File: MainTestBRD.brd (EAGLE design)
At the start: 100 x 62.2 mm, 24 parts, among them J1 COMPUTER-PERIPHERAL-POWERVERT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, U1 ATMEGA128-SMD

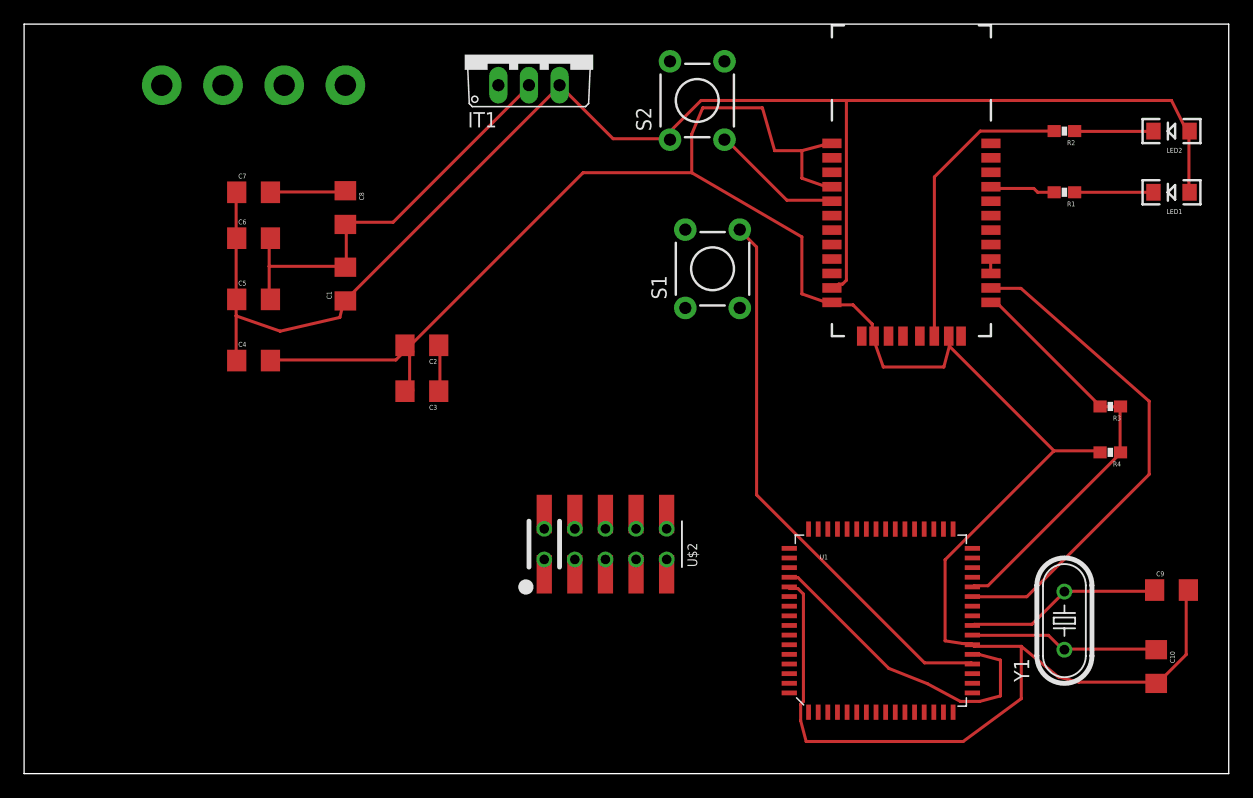
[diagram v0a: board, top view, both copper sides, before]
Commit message: other pinouts
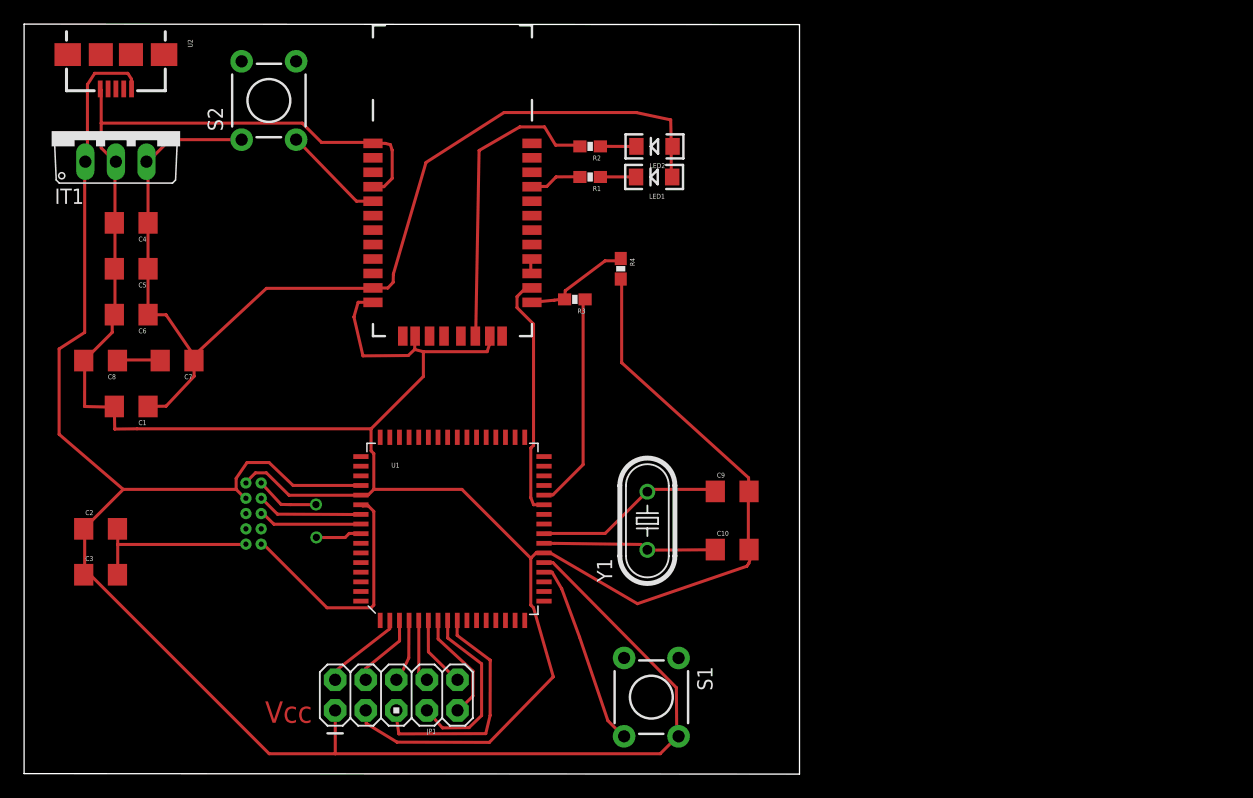
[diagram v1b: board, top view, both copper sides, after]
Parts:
- removed J1: COMPUTER-PERIPHERAL-POWERVERTICAL, SparkFun-Connectors:COMPUTER-PERIPHERAL-POWER
- removed U$2: JTAGICE3-CONNECTOR100MIL-SMD, con-jtagice3:JTAGICE3-100MIL-SMD
- added JP1: M05X2PTH, SparkFun-Connectors:AVR_ICSP
- added U$3: JTAGICE3-CONNECTOR50MIL-THT, con-jtagice3:JTAGICE3-50MIL
- added U2: (no value), SparkFun-Connectors:USB-AB-MICRO-SMD
- moved R3 45.3 mm to (45.7, 57.1)
- moved R4 43.4 mm to (49.5, 59.7), turned to 270 degrees
- moved LED1 43.0 mm to (52.3, 67.3)
- moved LED2 42.9 mm to (52.3, 69.8)
- moved R1 39.4 mm to (47.0, 67.3)
- moved R2 39.4 mm to (47.0, 69.8)
- moved U$1 38.1 mm to (35.6, 63.5)
- moved C9 37.4 mm to (58.8, 41.2)
- moved C10 36.5 mm to (58.8, 36.4), turned to 0 degrees
- moved U1 36.4 mm to (35.6, 38.1)
- moved S1 35.9 mm to (52.1, 24.1), turned to 270 degrees
- moved Y1 35.6 mm to (51.7, 38.8)
- moved S2 35.6 mm to (20.3, 73.7)
- moved IT1 34.9 mm to (7.62, 71.1)
- moved C2 30.7 mm to (6.35, 38.1), turned to 0 degrees
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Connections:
- new net N$10: JP1.10, U1.6
- new net N$11: JP1.8, U1.5
- new net N$12: JP1.6, U1.4
- new net N$13: JP1.4, U1.3
- new net N$14: JP1.2, U1.2
- new net N$15: JP1.9, U1.7
- new net N$16: JP1.7, U1.8
- new net N$17: JP1.5, U1.9
- new net N$3: R3.1, U1.28
- net BT_RX: no longer R3.1, U1.28
- net GND: now also JP1.3, U$3.P0, U$3.P2, U2.GND; no longer J1.GND
- net PF4: now also U$3.P1; no longer U$2.1
- net PF5: now also U$3.P5; no longer U$2.5
- net PF6: now also U$3.P3; no longer U$2.3
- net PF7: now also U$3.P9; no longer U$2.9
- net VCC: now also JP1.1, U$3.P4, U2.VBUS; no longer J1.5V, U$2.4
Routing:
- net VCC: track 30.6 -> 153.8 mm
- net VDD: track 128.7 -> 89.3 mm
- net RESET: track 46.3 -> 15.7 mm
- net BT_RX: track 35.1 -> 8.97 mm
- net BT_TX: track 41.6 -> 20.4 mm
- net PF7: track 0.00 -> 20.7 mm
- net N$17: track 0.00 -> 20.0 mm
- net N$3: track 0.00 -> 18.2 mm
- net N$16: track 0.00 -> 14.9 mm
- net N$15: track 0.00 -> 9.30 mm
- net PF5: track 0.00 -> 8.82 mm
- net PF6: track 0.00 -> 8.82 mm
- net N$14: track 0.00 -> 7.15 mm
- net N$13: track 0.00 -> 6.27 mm
- net N$10: track 0.00 -> 5.97 mm
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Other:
- board size 100 x 62.2 mm -> 64.4 x 62.3 mm
- board text added: "Vcc"
